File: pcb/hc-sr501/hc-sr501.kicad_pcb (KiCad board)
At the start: 2 copper layers, 35 x 25 mm, 35 parts, among them J1 Conector 3 pines, U1 BISS0001, U2 HT7133-1

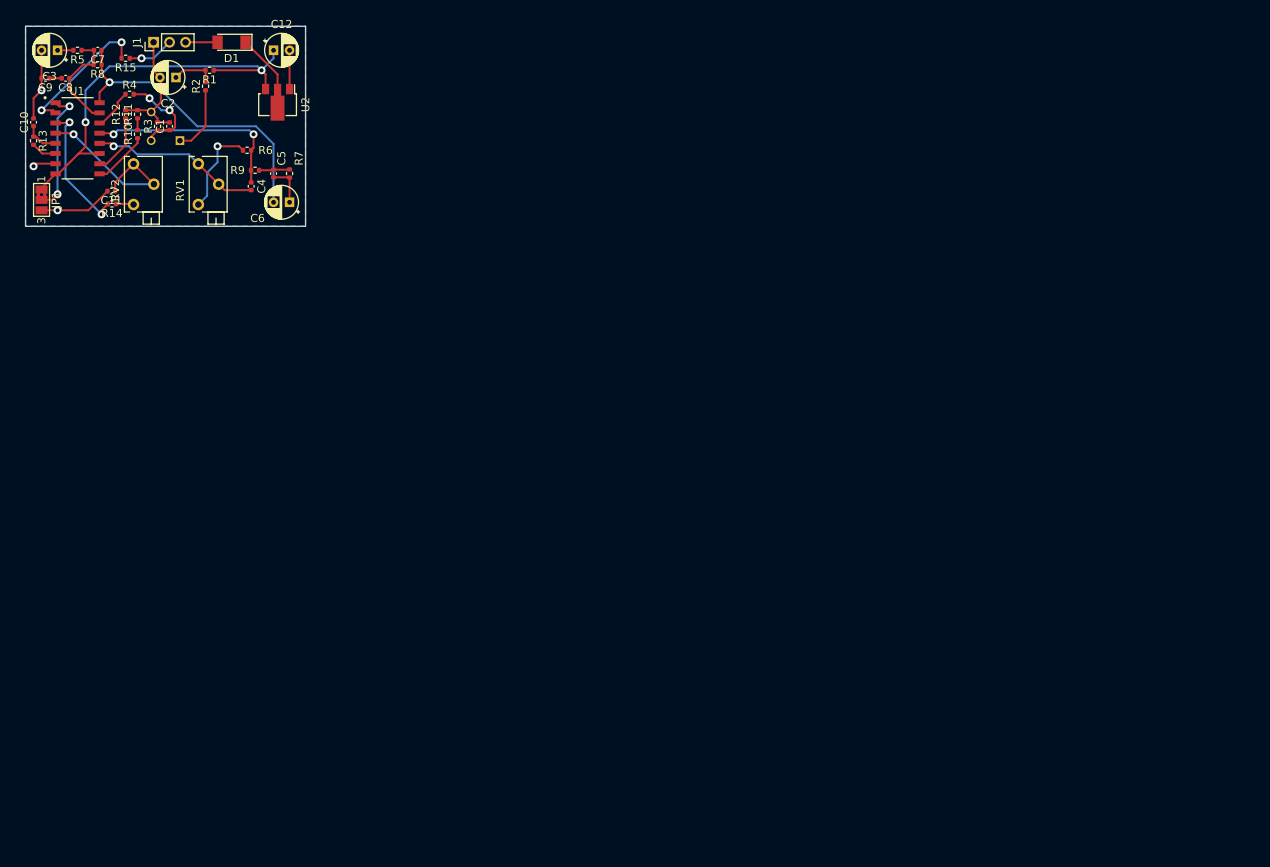
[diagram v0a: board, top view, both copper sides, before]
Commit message: Cambios de PCB
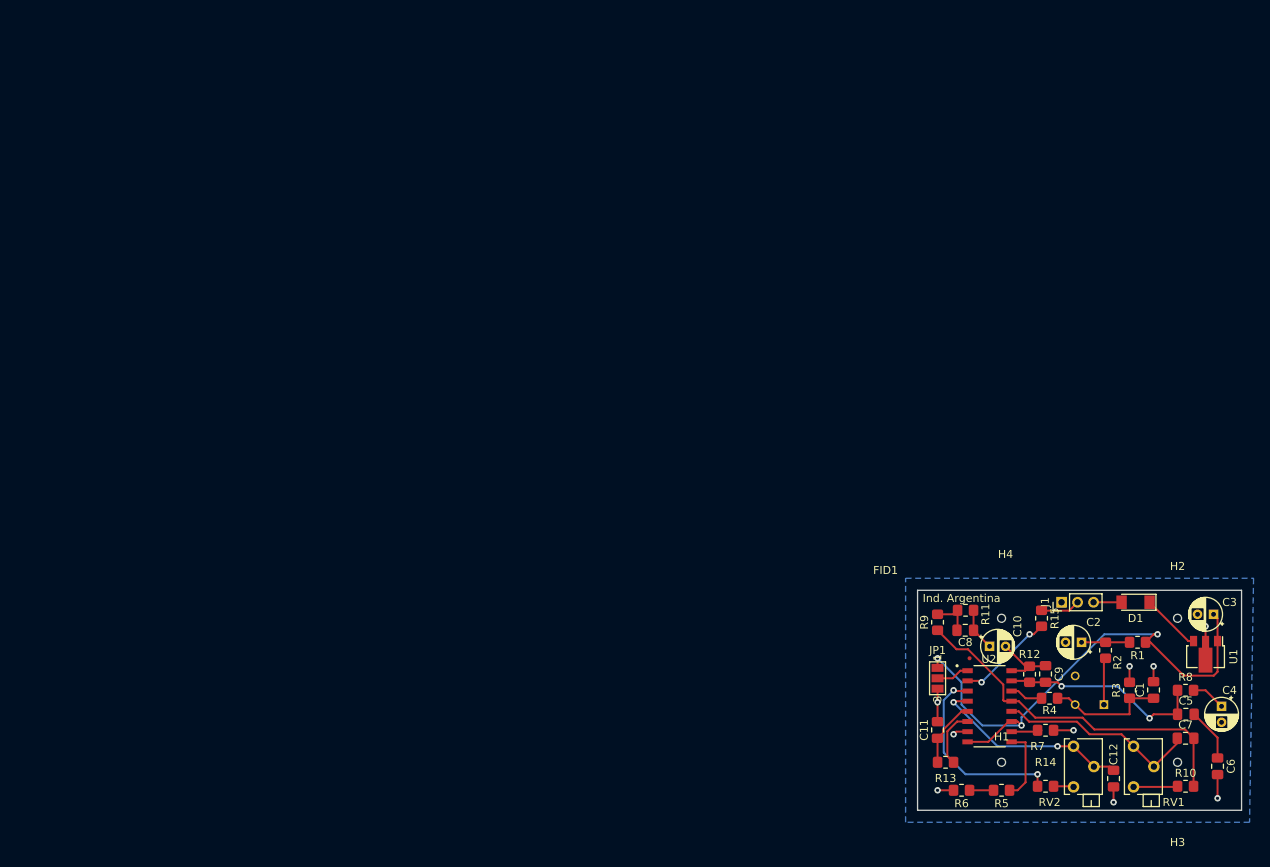
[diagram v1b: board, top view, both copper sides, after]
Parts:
- removed the C11 at (70.7, 60.6)
- removed the R12 at (72.5, 51.0)
- added C3: 22uF, Capacitor_THT:CP_Radial_D4.0mm_P2.00mm, F.Cu at (208.5, 113.5)
- added FID1: Fiducial, Fiducial:Fiducial_0.5mm_Mask1mm, F.Cu at (178.0, 119.0)
- added H1: MountingHole, myLib:MountingHole_1mm, F.Cu at (182.0, 132.0)
- added H2: MountingHole, myLib:MountingHole_1mm, F.Cu at (204.0, 114.0)
- added H3: MountingHole, myLib:MountingHole_1mm, F.Cu at (204.0, 132.0)
- added H4: MountingHole, myLib:MountingHole_1mm, F.Cu at (182.0, 114.0)
- added R7: 1M, Resistor_SMD:R_0805_2012Metric_Pad1.20x1.40mm_HandSolder, F.Cu at (187.5, 128.0)
- C1: footprint Capacitor_SMD:C_0402_1005Metric -> Capacitor_SMD:C_0805_2012Metric_Pad1.18x1.45mm_HandSolder
- C11: renamed from C10; footprint Capacitor_SMD:C_0402_1005Metric -> Capacitor_SMD:C_0805_2012Metric_Pad1.18x1.45mm_HandSolder
- C12: value 22uF -> 10nF; footprint Capacitor_THT:CP_Radial_D4.0mm_P2.00mm -> Capacitor_SMD:C_0805_2012Metric_Pad1.18x1.45mm_HandSolder
- C5: renamed from C8; footprint Capacitor_SMD:C_0402_1005Metric -> Capacitor_SMD:C_0805_2012Metric_Pad1.18x1.45mm_HandSolder
- C6: renamed from C9; footprint Capacitor_SMD:C_0402_1005Metric -> Capacitor_SMD:C_0805_2012Metric_Pad1.18x1.45mm_HandSolder
- C7: renamed from C4; footprint Capacitor_SMD:C_0402_1005Metric -> Capacitor_SMD:C_0805_2012Metric_Pad1.18x1.45mm_HandSolder
- C8: renamed from C5; footprint Capacitor_SMD:C_0402_1005Metric -> Capacitor_SMD:C_0805_2012Metric_Pad1.18x1.45mm_HandSolder
- C9: renamed from C7; footprint Capacitor_SMD:C_0402_1005Metric -> Capacitor_SMD:C_0805_2012Metric_Pad1.18x1.45mm_HandSolder
- D1: value D_ALT -> 1N5819
- JP1: footprint Jumper:SolderJumper-3_P1.3mm_Bridged2Bar12_Pad1.0x1.5mm_NumberLabels -> Jumper:SolderJumper-3_P1.3mm_Open_Pad1.0x1.5mm_NumberLabels
- R1, R13, R14, R15, R2, R3, R4, R9: footprint Resistor_SMD:R_0402_1005Metric -> Resistor_SMD:R_0805_2012Metric_Pad1.20x1.40mm_HandSolder
- R10: renamed from R6; footprint Resistor_SMD:R_0402_1005Metric -> Resistor_SMD:R_0805_2012Metric_Pad1.20x1.40mm_HandSolder
- R11: renamed from R7; footprint Resistor_SMD:R_0402_1005Metric -> Resistor_SMD:R_0805_2012Metric_Pad1.20x1.40mm_HandSolder
- R12: renamed from R8; footprint Resistor_SMD:R_0402_1005Metric -> Resistor_SMD:R_0805_2012Metric_Pad1.20x1.40mm_HandSolder
- R5: renamed from R10; footprint Resistor_SMD:R_0402_1005Metric -> Resistor_SMD:R_0805_2012Metric_Pad1.20x1.40mm_HandSolder
- R6: renamed from R11; footprint Resistor_SMD:R_0402_1005Metric -> Resistor_SMD:R_0805_2012Metric_Pad1.20x1.40mm_HandSolder
- R8: renamed from R5; footprint Resistor_SMD:R_0402_1005Metric -> Resistor_SMD:R_0805_2012Metric_Pad1.20x1.40mm_HandSolder
- U1: value BISS0001 -> L78L33_SOT89; footprint myLib:SOIC127P600X180-16N -> Package_TO_SOT_SMD:SOT-89-3
- U2: value HT7133-1 -> BISS0001; footprint Package_TO_SOT_SMD:SOT-89-3 -> myLib:SOIC127P600X180-16N
- moved C6 169.9 mm to (209.0, 132.5), turned to 270 degrees
- moved C4 167.0 mm to (209.5, 125.0), turned to 270 degrees
- moved C5 161.0 mm to (205.0, 126.0), turned to 0 degrees
- moved R8 160.0 mm to (205.0, 123.0), turned to 0 degrees
- moved U1 155.1 mm to (207.5, 118.5), turned to 270 degrees
- moved C9 141.8 mm to (187.5, 121.0), turned to 270 degrees
- moved C1 141.8 mm to (201.0, 123.0)
- moved R10 141.7 mm to (205.0, 135.0)
- moved R3 140.5 mm to (198.0, 123.0)
- moved R12 139.2 mm to (185.5, 121.0), turned to 270 degrees
- moved C12 139.0 mm to (196.0, 134.0), turned to 270 degrees
- moved RV2 138.2 mm to (191.0, 130.0)
- moved R13 138.0 mm to (175.0, 132.0), turned to 0 degrees
- moved RV1 137.7 mm to (198.5, 130.0)
- moved R4 137.6 mm to (188.0, 124.0)
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- renumbered C6 to C10, C3 to C4
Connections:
- C11 pad 1: Net-(C10-Pad1) (its old number) -> Net-(C11-Pad1)
- C12 pad 1: +3V3 -> Net-(C12-Pad1)
- R13 pad 1: Net-(C10-Pad1) (its old number) -> Net-(C11-Pad1)
- R5 pad 1: Net-(R10-Pad1) (its old number) -> Net-(R5-Pad1)
- RV2 pad 1: Net-(C11-Pad1) -> Net-(C12-Pad1)
- RV2 pad 2: Net-(C11-Pad1) -> Net-(C12-Pad1)
- U1 pad 1: Net-(JP1-Pad2) -> +3V3
- U1 pad 2: Net-(R15-Pad2) -> GND
- U1 pad 3: Net-(R14-Pad2) -> Net-(D1-Pad1)
- U2 pad 1: GND -> Net-(JP1-Pad2)
- U2 pad 2: Net-(D1-Pad1) -> Net-(R15-Pad2)
- U2 pad 3: +3V3 -> Net-(R14-Pad2)
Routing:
- net /1OUT: track 38.5 -> 8.55 mm, vias 1 -> 0
- net Net-(C12-Pad1): track 0.00 -> 25.3 mm, vias 0 -> 2
- net GND: track 42.3 -> 20.3 mm, vias 3 -> 9
- net /2IN-: track 25.9 -> 44.8 mm, vias 2 -> 0
- net +3V3: track 52.8 -> 67.7 mm, vias 2 -> 3
- net Net-(C11-Pad1): track 22.9 -> 8.35 mm, vias 1 -> 0
- net /1IN-: track 13.5 -> 25.9 mm, vias 0 -> 2
- net Net-(JP1-Pad2): track 15.8 -> 4.14 mm, vias 2 -> 0
- net Net-(R5-Pad1): track 0.00 -> 9.69 mm
- net Net-(R12-Pad1): track 7.54 -> 0.00 mm
- net Net-(R14-Pad2): track 17.0 -> 24.4 mm
- net Net-(R10-Pad1) (its old number): track 6.94 -> 0.00 mm
- net Net-(R10-Pad1): track 11.7 -> 5.53 mm, vias 1 -> 0
- net Net-(C5-Pad2): track 1.56 -> 6.67 mm
- net Net-(R15-Pad2): track 17.4 -> 12.7 mm
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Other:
- board size 35 x 25 mm -> 40.5 x 27.5 mm
- rule pad_to_mask_clearance: 0 -> 0.07
- rule trace_min: 0.2 -> 0.25
- rule via_min_size: 0.4 -> 0.6
- board text added: "Ancho de pistas: 0.25 mm"
- board text added: "Fabricante: Mayer PCB (10 mils) Terminacion HASL"
- board text added: "Ind. Argentina"
- board text added: "Margen: 0,3 mm Grilla: 0,5 mm"
- board text added: "Réplica HC-SR501 Ind. Argentina"
- board text added: "Vias: 0,40 mm Pad: 0,80 mm"
